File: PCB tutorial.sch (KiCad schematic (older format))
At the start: 5 parts

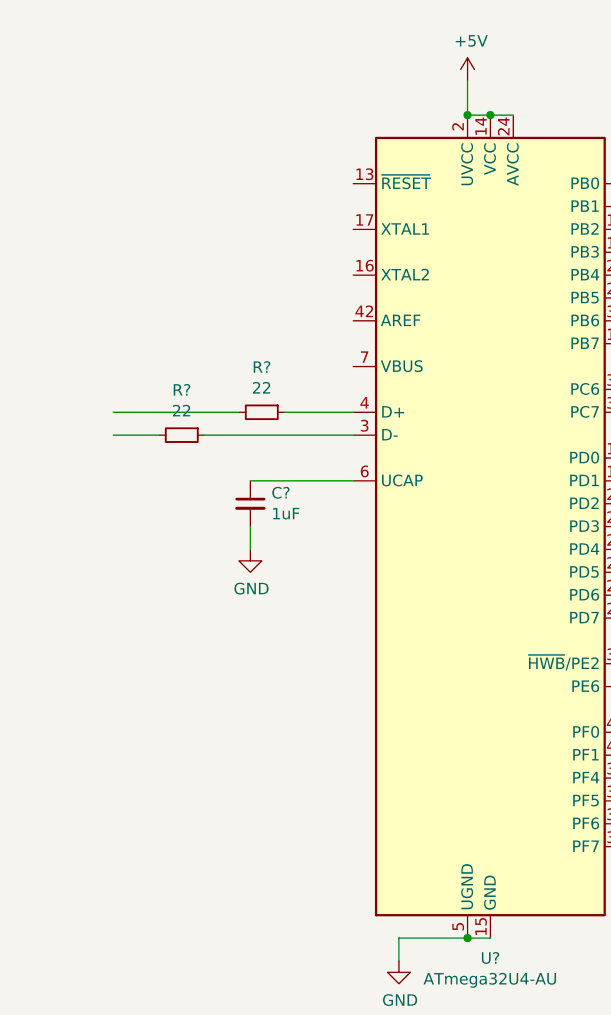
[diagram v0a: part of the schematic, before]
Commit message: MCU zone completed
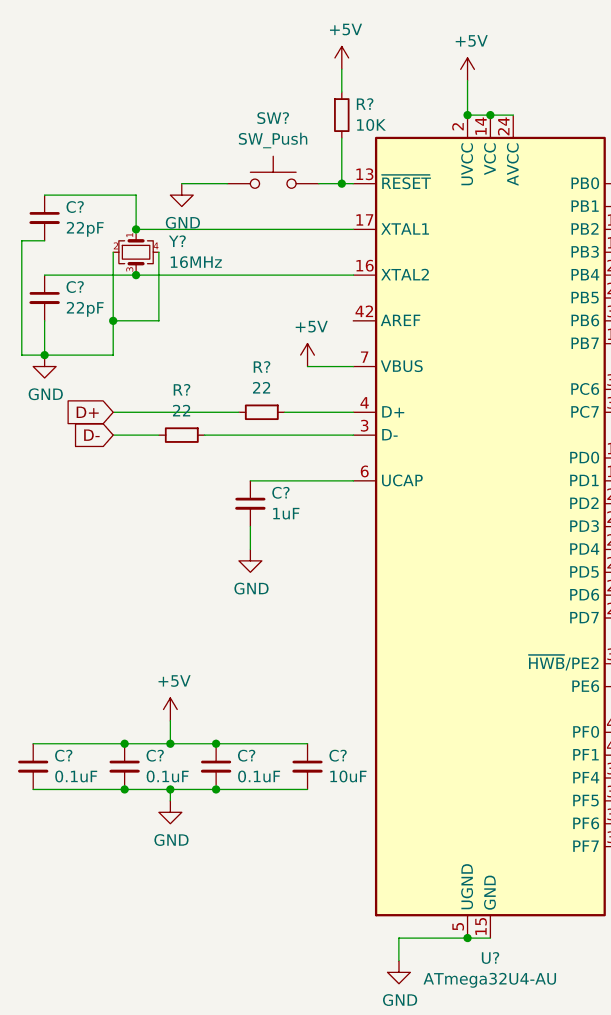
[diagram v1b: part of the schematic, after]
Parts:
- added C? (x3): 0.1uF, symbol Device:C_Small
- added C?: 10uF, symbol Device:C_Small
- added C? (x2): 22pF, symbol Device:C_Small
- added R?: 10K, symbol Device:R_Small
- added SW?: SW_Push, symbol Switch:SW_Push
- added Y?: 16MHz, symbol Device:Crystal_GND24_Small
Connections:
- net labels added: D+, D-
- wire segments 15 -> 45
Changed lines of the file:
@@
 Wire Wire Line
 	1500 3100 1500 3200
+$Comp
+L Device:C_Small C?
+U 1 1 60FB5F7C
+P 950 4150
+F 0 "C?" H 1042 4196 50  0000 L CNN
+F 1 "0.1uF" H 1042 4105 50  0000 L CNN
+F 2 "" H 950 4150 50  0001 C CNN
+F 3 "~" H 950 4150 50  0001 C CNN
+	1    950  4150
+	1    0    0    -1
+$EndComp
+$Comp
+L Device:C_Small C?
+U 1 1 60FB722C
+P 1350 4150
+F 0 "C?" H 1442 4196 50  0000 L CNN
+F 1 "0.1uF" H 1442 4105 50  0000 L CNN
+F 2 "" H 1350 4150 50  0001 C CNN
+F 3 "~" H 1350 4150 50  0001 C CNN
+	1    1350 4150
+	1    0    0    -1
+$EndComp
+$Comp
+L Device:C_Small C?
+U 1 1 60FB7B19
+P 550 4150
+F 0 "C?" H 642 4196 50  0000 L CNN
+F 1 "0.1uF" H 642 4105 50  0000 L CNN
+F 2 "" H 550 4150 50  0001 C CNN
+F 3 "~" H 550 4150 50  0001 C CNN
+	1    550  4150
+	1    0    0    -1
+$EndComp
+$Comp
+L Device:C_Small C?
+U 1 1 60FBA18D
+P 1750 4150
+F 0 "C?" H 1842 4196 50  0000 L CNN
+F 1 "10uF" H 1842 4105 50  0000 L CNN
+F 2 "" H 1750 4150 50  0001 C CNN
+F 3 "~" H 1750 4150 50  0001 C CNN
+	1    1750 4150
+	1    0    0    -1
+$EndComp
+$Comp
+L power:+5V #PWR?
+U 1 1 60FBB0DB
+P 1150 3950
+F 0 "#PWR?" H 1150 3800 50  0001 C CNN
+F 1 "+5V" H 1165 4123 50  0000 C CNN
+F 2 "" H 1150 3950 50  0001 C CNN
+F 3 "" H 1150 3950 50  0001 C CNN
+	1    1150 3950
+	1    0    0    -1
+$EndComp
+$Comp
+L power:GND #PWR?
+U 1 1 60FBBF77
+P 1150 4300
+F 0 "#PWR?" H 1150 4050 50  0001 C CNN
+F 1 "GND" H 1155 4127 50  0000 C CNN
+F 2 "" H 1150 4300 50  0001 C CNN
+F 3 "" H 1150 4300 50  0001 C CNN
+	1    1150 4300
+	1    0    0    -1
+$EndComp
+Wire Wire Line
+	550  4050 950  4050
+Wire Wire Line
+	950  4050 1150 4050
+Connection ~ 950  4050
+Wire Wire Line
+	1350 4050 1750 4050
+Connection ~ 1350 4050
+Wire Wire Line
+	1150 3950 1150 4050
+Connection ~ 1150 4050
+Wire Wire Line
+	1150 4050 1350 4050
+Wire Wire Line
+	550  4250 950  4250
+Wire Wire Line
+	950  4250 1150 4250
+Connection ~ 950  4250
+Wire Wire Line
+	1350 4250 1750 4250
+Connection ~ 1350 4250
+Wire Wire Line
+	1150 4250 1150 4300
+Connection ~ 1150 4250
+Wire Wire Line
+	1150 4250 1350 4250
+$Comp
+L power:+5V #PWR?
+U 1 1 60FBF19C
+P 1750 2400
+F 0 "#PWR?" H 1750 2250 50  0001 C CNN
+F 1 "+5V" H 1765 2573 50  0000 C CNN
+F 2 "" H 1750 2400 50  0001 C CNN
+F 3 "" H 1750 2400 50  0001 C CNN
+	1    1750 2400
+	1    0    0    -1
+$EndComp
+Wire Wire Line
+	1750 2400 1950 2400
+$Comp
+L Device:Crystal_GND24_Small Y?
+U 1 1 60FC04F2
+P 1000 1900
+F 0 "Y?" V 954 2044 50  0000 L CNN
+F 1 "16MHz" V 1045 2044 50  0000 L CNN
+F 2 "" H 1000 1900 50  0001 C CNN
+F 3 "~" H 1000 1900 50  0001 C CNN
+	1    1000 1900
+	0    1    1    0
+$EndComp
+Wire Wire Line
+	1000 1800 1950 1800
+Wire Wire Line
+	1000 2000 1950 2000
+$Comp
+L Device:C_Small C?
+U 1 1 60FC39C0
+P 600 1750
+F 0 "C?" H 692 1796 50  0000 L CNN
+F 1 "22pF" H 692 1705 50  0000 L CNN
+F 2 "" H 600 1750 50  0001 C CNN
+F 3 "~" H 600 1750 50  0001 C CNN
+	1    600  1750
+	1    0    0    -1
+$EndComp
+$Comp
+L Device:C_Small C?
+U 1 1 60FC4DBC
+P 600 2100
+F 0 "C?" H 692 2146 50  0000 L CNN
+F 1 "22pF" H 692 2055 50  0000 L CNN
+F 2 "" H 600 2100 50  0001 C CNN
+F 3 "~" H 600 2100 50  0001 C CNN
+	1    600  2100
+	1    0    0    -1
+$EndComp
+$Comp
+L power:GND #PWR?
+U 1 1 60FC61FA
+P 600 2350
+F 0 "#PWR?" H 600 2100 50  0001 C CNN
+F 1 "GND" H 605 2177 50  0000 C CNN
+F 2 "" H 600 2350 50  0001 C CNN
+F 3 "" H 600 2350 50  0001 C CNN
+	1    600  2350
+	1    0    0    -1
+$EndComp
+Wire Wire Line
+	1000 1800 1000 1650
+Wire Wire Line
+	1000 1650 600  1650
+Connection ~ 1000 1800
+Wire Wire Line
+	1000 2000 600  2000
+Connection ~ 1000 2000
+Wire Wire Line
+	600  2350 900  2350
+Wire Wire Line
+	900  2350 900  2200
+Wire Wire Line
+	1100 1900 1100 2200
+Wire Wire Line
+	1100 2200 900  2200
+Connection ~ 900  2200
+Wire Wire Line
+	900  2200 900  1900
+Wire Wire Line
+	600  2200 600  2350
+Connection ~ 600  2350
+Wire Wire Line
+	600  1850 500  1850
+Wire Wire Line
+	500  1850 500  2350
+Wire Wire Line
+	500  2350 600  2350
+$Comp
+L Switch:SW_Push SW?
+U 1 1 60FCB650
+P 1600 1600
+F 0 "SW?" H 1600 1885 50  0000 C CNN
+F 1 "SW_Push" H 1600 1794 50  0000 C CNN
+F 2 "" H 1600 1800 50  0001 C CNN
+F 3 "~" H 1600 1800 50  0001 C CNN
+	1    1600 1600
+	1    0    0    -1
+$EndComp
+Wire Wire Line
+	1800 1600 1900 1600
+$Comp
+L power:GND #PWR?
+U 1 1 60FCD847
+P 1200 1600
+F 0 "#PWR?" H 1200 1350 50  0001 C CNN
+F 1 "GND" H 1205 1427 50  0000 C CNN
+F 2 "" H 1200 1600 50  0001 C CNN
+F 3 "" H 1200 1600 50  0001 C CNN
+	1    1200 1600
+	1    0    0    -1
+$EndComp
+Wire Wire Line
+	1200 1600 1400 1600
+$Comp
+L Device:R_Small R?
+U 1 1 60FCF027
+P 1900 1300
+F 0 "R?" H 1959 1346 50  0000 L CNN
+F 1 "10K" H 1959 1255 50  0000 L CNN
+F 2 "" H 1900 1300 50  0001 C CNN
+F 3 "~" H 1900 1300 50  0001 C CNN
+	1    1900 1300
+	1    0    0    -1
+$EndComp
+$Comp
+L power:+5V #PWR?
+U 1 1 60FD05C9
+P 1900 1100
+F 0 "#PWR?" H 1900 950 50  0001 C CNN
+F 1 "+5V" H 1915 1273 50  0000 C CNN
+F 2 "" H 1900 1100 50  0001 C CNN
+F 3 "" H 1900 1100 50  0001 C CNN
+	1    1900 1100
+	1    0    0    -1
+$EndComp
+Wire Wire Line
+	1900 1400 1900 1600
+Connection ~ 1900 1600
+Wire Wire Line
+	1900 1600 1950 1600
+Wire Wire Line
+	1900 1200 1900 1100
+Text GLabel 900  2600 0    50   Input ~ 0
+D+
+Text GLabel 900  2700 0    50   Input ~ 0
+D-
 $EndSCHEMATC

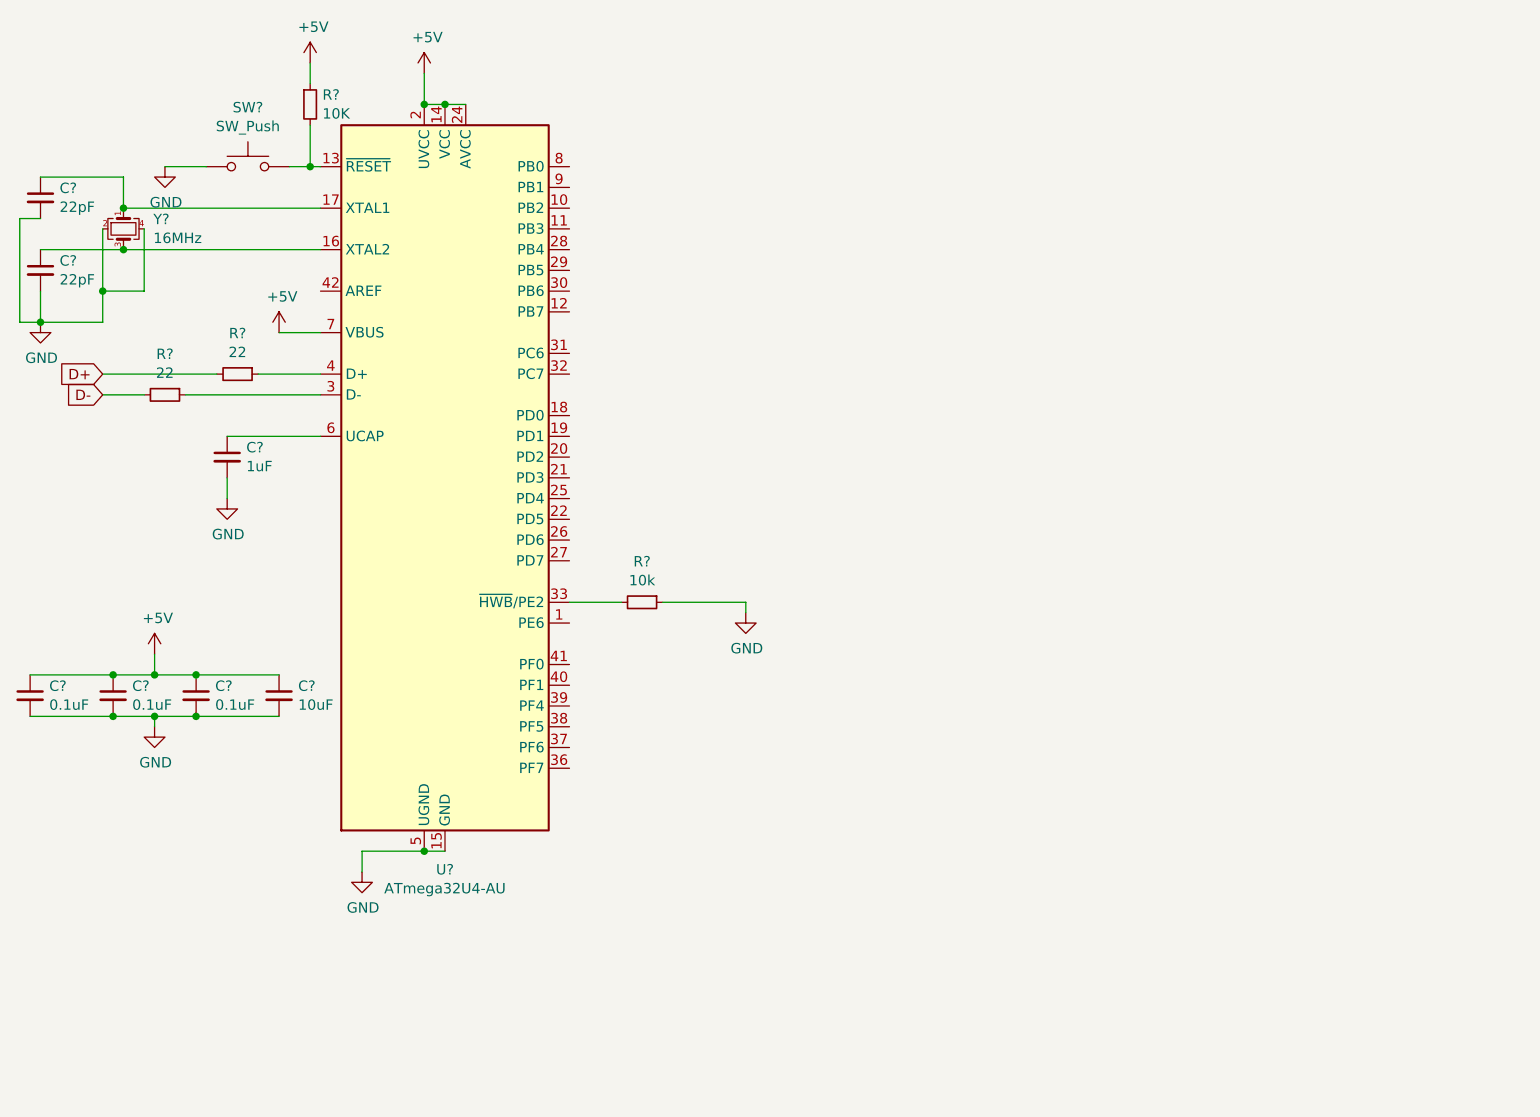
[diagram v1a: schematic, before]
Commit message: Switch Schematic
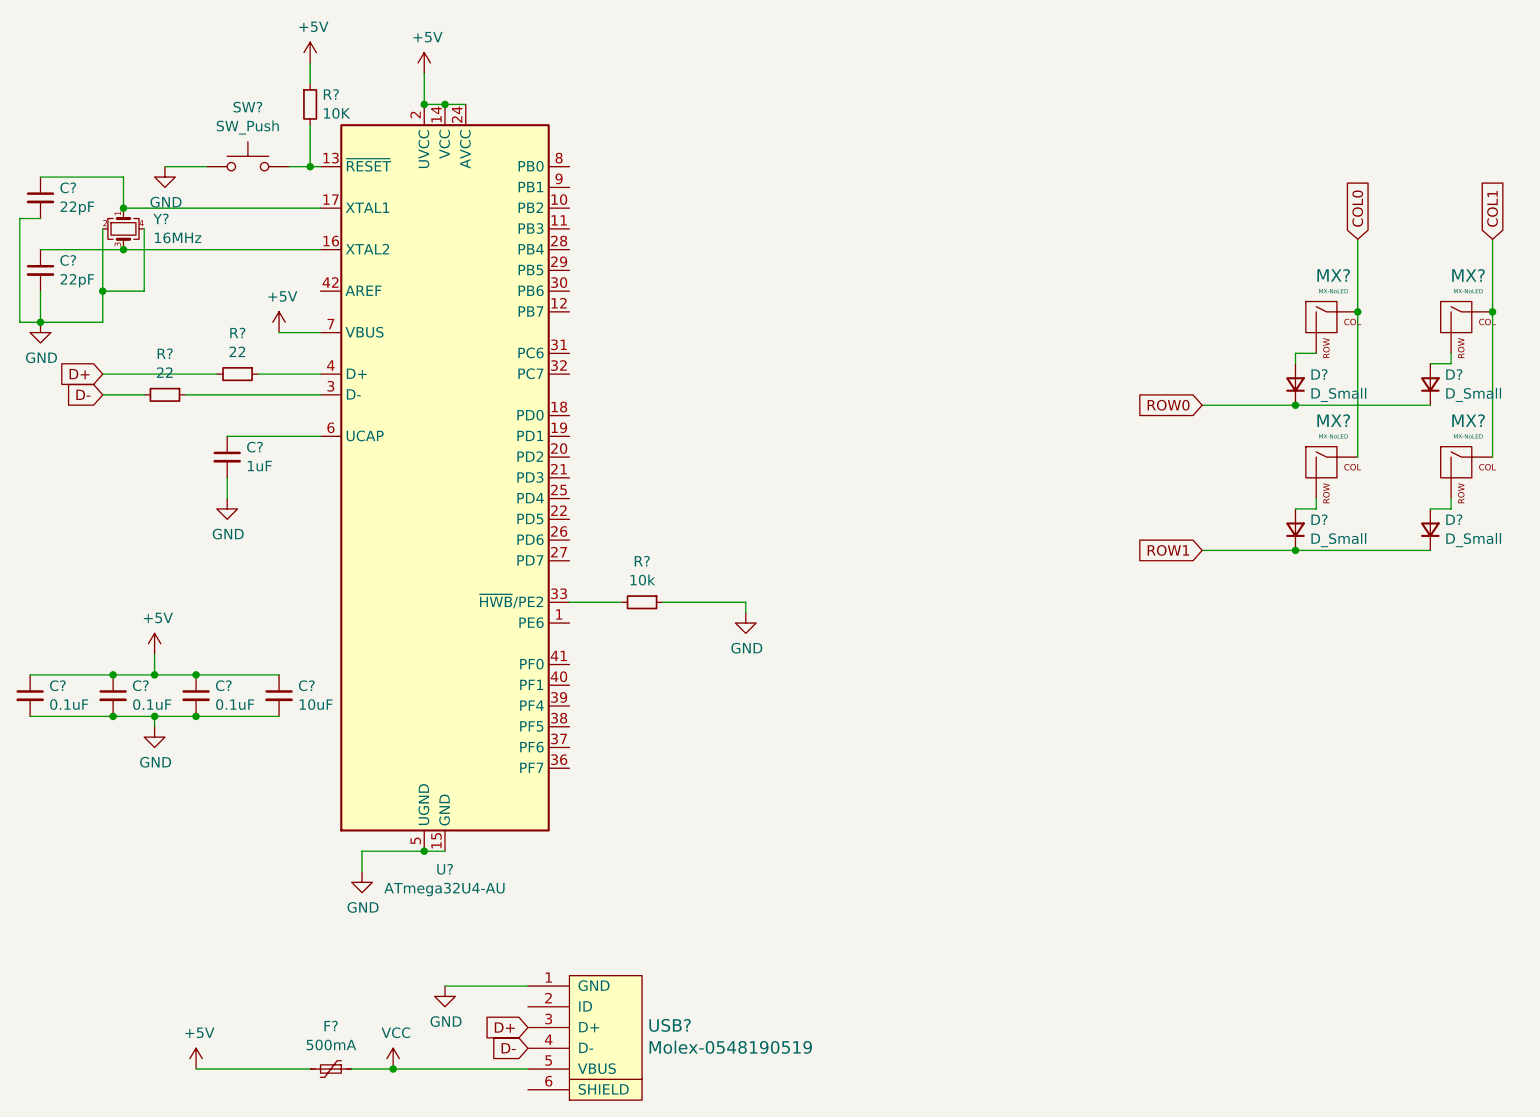
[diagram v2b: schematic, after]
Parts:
- added D? (x4): D_Small, symbol Device:D_Small
- added F?: 500mA, symbol Device:Polyfuse_Small
- added MX? (x4): MX-NoLED, symbol MX_Alps_Hybrid:MX-NoLED
- added USB?: Molex-0548190519, symbol random-keyboard-parts:Molex-0548190519
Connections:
- net +5V: now also F?.2
- net D+: now also USB?.3 (D+)
- net D-: now also USB?.4 (D-)
- net GND: now also USB?.1 (GND)
- new net: D?.2 (A), MX?.2 (ROW) (x4)
- new net COL0: MX?.1 (COL), MX?.1 (COL)
- new net COL1: MX?.1 (COL), MX?.1 (COL)
- new net ROW0: D?.1 (K), D?.1 (K)
- new net ROW1: D?.1 (K), D?.1 (K)
- new net VCC: F?.1, USB?.5 (VBUS)
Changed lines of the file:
@@
 Text GLabel 900  2700 0    50   Input ~ 0
 D-
+$Comp
+L random-keyboard-parts:Molex-0548190519 USB?
+U 1 1 60FD3794
+P 3250 5750
+F 0 "USB?" V 3242 6028 60  0000 L CNN
+F 1 "Molex-0548190519" V 3348 6028 60  0000 L CNN
+F 2 "" H 3250 5750 60  0001 C CNN
+F 3 "" H 3250 5750 60  0001 C CNN
+	1    3250 5750
+	0    1    1    0
+$EndComp
+$Comp
+L Device:Polyfuse_Small F?
+U 1 1 60FD6C5F
+P 2000 5950
+F 0 "F?" V 1795 5950 50  0000 C CNN
+F 1 "500mA" V 1886 5950 50  0000 C CNN
+F 2 "" H 2050 5750 50  0001 L CNN
+F 3 "~" H 2000 5950 50  0001 C CNN
+	1    2000 5950
+	0    1    1    0
+$EndComp
+$Comp
+L power:+5V #PWR?
+U 1 1 60FD8EE3
+P 1350 5950
+F 0 "#PWR?" H 1350 5800 50  0001 C CNN
+F 1 "+5V" H 1365 6123 50  0000 C CNN
+F 2 "" H 1350 5950 50  0001 C CNN
+F 3 "" H 1350 5950 50  0001 C CNN
+	1    1350 5950
+	1    0    0    -1
+$EndComp
+Wire Wire Line
+	1350 5950 1900 5950
+Wire Wire Line
+	2100 5950 2300 5950
+$Comp
+L power:VCC #PWR?
+U 1 1 60FDBFB6
+P 2300 5950
+F 0 "#PWR?" H 2300 5800 50  0001 C CNN
+F 1 "VCC" H 2315 6123 50  0000 C CNN
+F 2 "" H 2300 5950 50  0001 C CNN
+F 3 "" H 2300 5950 50  0001 C CNN
+	1    2300 5950
+	1    0    0    -1
+$EndComp
+Connection ~ 2300 5950
+Wire Wire Line
+	2300 5950 2950 5950
+Text GLabel 2950 5750 0    50   Input ~ 0
+D+
+Text GLabel 2950 5850 0    50   Input ~ 0
+D-
+$Comp
+L power:GND #PWR?
+U 1 1 60FDE1F9
+P 2550 5550
+F 0 "#PWR?" H 2550 5300 50  0001 C CNN
+F 1 "GND" H 2555 5377 50  0000 C CNN
+F 2 "" H 2550 5550 50  0001 C CNN
+F 3 "" H 2550 5550 50  0001 C CNN
+	1    2550 5550
+	1    0    0    -1
+$EndComp
+Wire Wire Line
+	2550 5550 2950 5550
+$Comp
+L MX_Alps_Hybrid:MX-NoLED MX?
+U 1 1 60FE0262
+P 6800 2350
+F 0 "MX?" H 6833 2573 60  0000 C CNN
+F 1 "MX-NoLED" H 6833 2499 20  0000 C CNN
+F 2 "" H 6175 2325 60  0001 C CNN
+F 3 "" H 6175 2325 60  0001 C CNN
+	1    6800 2350
+	1    0    0    -1
+$EndComp
+$Comp
+L Device:D_Small D?
+U 1 1 60FE1176
+P 6650 2650
+F 0 "D?" V 6696 2580 50  0000 R CNN
+F 1 "D_Small" V 6605 2580 50  0000 R CNN
+F 2 "" V 6650 2650 50  0001 C CNN
+F 3 "~" V 6650 2650 50  0001 C CNN
+	1    6650 2650
+	0    -1   -1   0
+$EndComp
+Wire Wire Line
+	6750 2500 6650 2500
+Wire Wire Line
+	6650 2500 6650 2550
+$Comp
+L MX_Alps_Hybrid:MX-NoLED MX?
+U 1 1 60FE583E
+P 7450 2350
+F 0 "MX?" H 7483 2573 60  0000 C CNN
+F 1 "MX-NoLED" H 7483 2499 20  0000 C CNN
+F 2 "" H 6825 2325 60  0001 C CNN
+F 3 "" H 6825 2325 60  0001 C CNN
+	1    7450 2350
+	1    0    0    -1
+$EndComp
+$Comp
+L Device:D_Small D?
+U 1 1 60FE656A
+P 7300 2650
+F 0 "D?" V 7346 2580 50  0000 R CNN
+F 1 "D_Small" V 7255 2580 50  0000 R CNN
+F 2 "" V 7300 2650 50  0001 C CNN
+F 3 "~" V 7300 2650 50  0001 C CNN
+	1    7300 2650
+	0    -1   -1   0
+$EndComp
+Wire Wire Line
+	7300 2550 7400 2550
+Wire Wire Line
+	7400 2550 7400 2500
+$Comp
+L MX_Alps_Hybrid:MX-NoLED MX?
+U 1 1 60FE84C8
+P 7450 3050
+F 0 "MX?" H 7483 3273 60  0000 C CNN
+F 1 "MX-NoLED" H 7483 3199 20  0000 C CNN
+F 2 "" H 6825 3025 60  0001 C CNN
+F 3 "" H 6825 3025 60  0001 C CNN
+	1    7450 3050
+	1    0    0    -1
+$EndComp
+$Comp
+L Device:D_Small D?
+U 1 1 60FE943D
+P 7300 3350
+F 0 "D?" V 7346 3280 50  0000 R CNN
+F 1 "D_Small" V 7255 3280 50  0000 R CNN
+F 2 "" V 7300 3350 50  0001 C CNN
+F 3 "~" V 7300 3350 50  0001 C CNN
+	1    7300 3350
+	0    -1   -1   0
+$EndComp
+$Comp
+L MX_Alps_Hybrid:MX-NoLED MX?
+U 1 1 60FEA45C
+P 6800 3050
+F 0 "MX?" H 6833 3273 60  0000 C CNN
+F 1 "MX-NoLED" H 6833 3199 20  0000 C CNN
+F 2 "" H 6175 3025 60  0001 C CNN
+F 3 "" H 6175 3025 60  0001 C CNN
+	1    6800 3050
+	1    0    0    -1
+$EndComp
+$Comp
+L Device:D_Small D?
+U 1 1 60FEE199
+P 6650 3350
+F 0 "D?" V 6696 3280 50  0000 R CNN
+F 1 "D_Small" V 6605 3280 50  0000 R CNN
+F 2 "" V 6650 3350 50  0001 C CNN
+F 3 "~" V 6650 3350 50  0001 C CNN
+	1    6650 3350
+	0    -1   -1   0
+$EndComp
+Wire Wire Line
+	6750 3200 6750 3250
+Wire Wire Line
+	6750 3250 6650 3250
+Wire Wire Line
+	7400 3200 7400 3250
+Wire Wire Line
+	7400 3250 7300 3250
+Wire Wire Line
+	7300 2750 6650 2750
+Wire Wire Line
+	6650 2750 6200 2750
+Connection ~ 6650 2750
+Wire Wire Line
+	7300 3450 6650 3450
+Wire Wire Line
+	6650 3450 6200 3450
+Connection ~ 6650 3450
+Wire Wire Line
+	6950 3000 6950 2300
+Wire Wire Line
+	6950 2300 6950 1950
+Connection ~ 6950 2300
+Wire Wire Line
+	7600 3000 7600 2300
+Wire Wire Line
+	7600 2300 7600 1950
+Connection ~ 7600 2300
+Text GLabel 6200 2750 0    50   Input ~ 0
+ROW0
+Text GLabel 6200 3450 0    50   Input ~ 0
+ROW1
+Text GLabel 6950 1950 1    50   Input ~ 0
+COL0
+Text GLabel 7600 1950 1    50   Input ~ 0
+COL1
 $EndSCHEMATC
